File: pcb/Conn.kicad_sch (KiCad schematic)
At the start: 5 parts

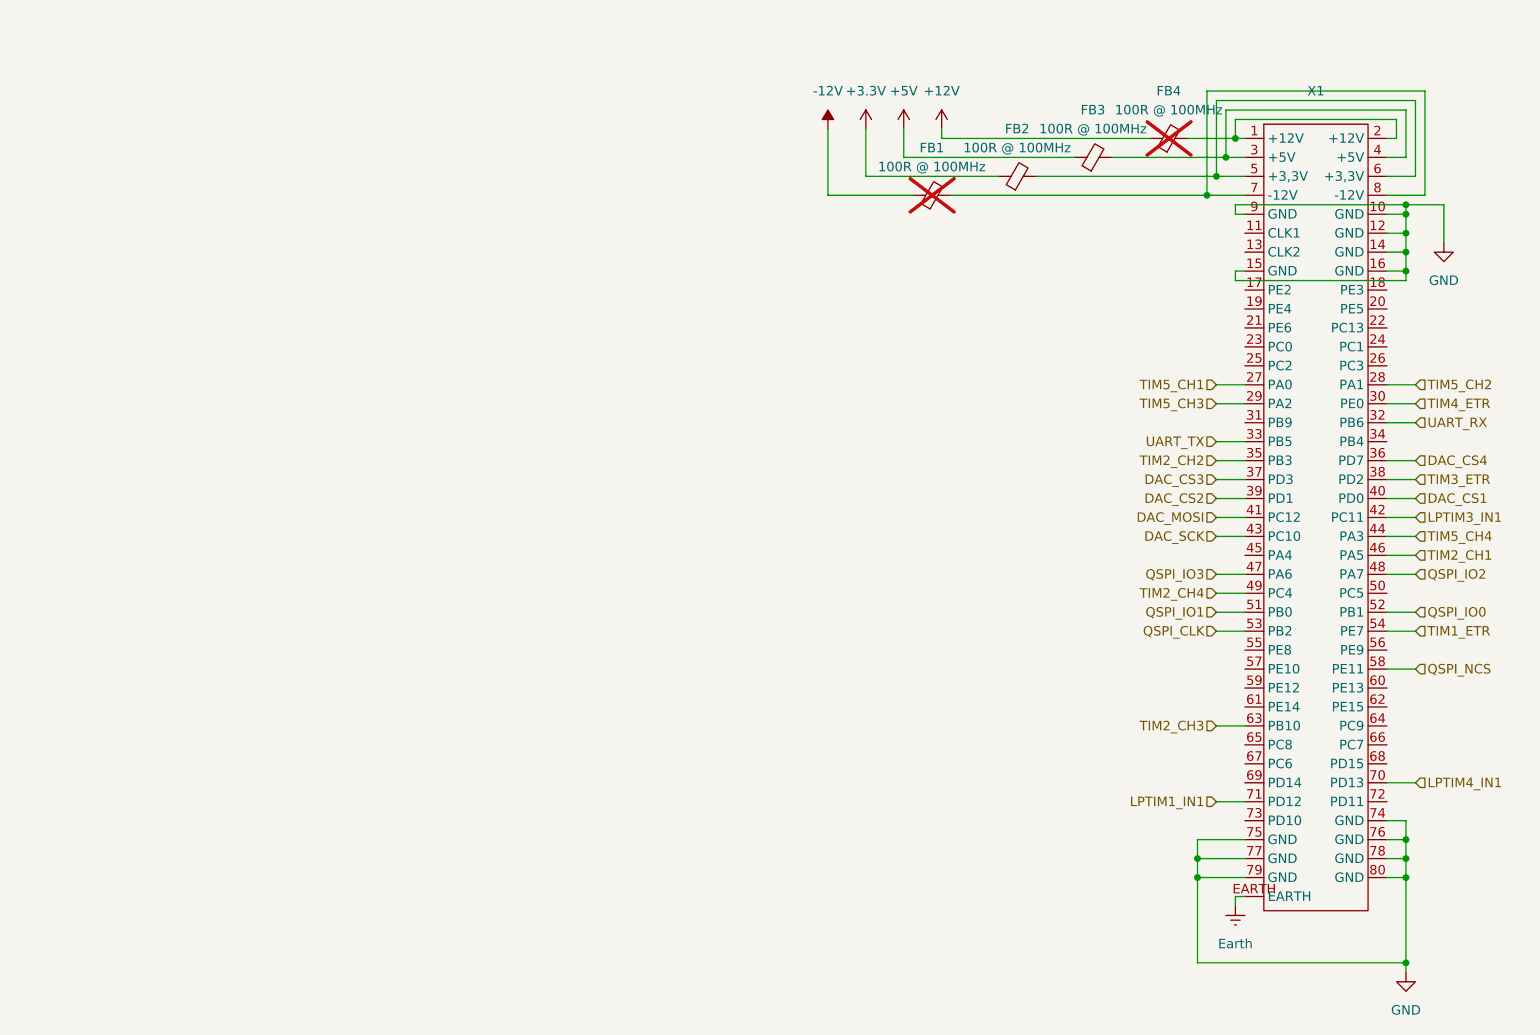
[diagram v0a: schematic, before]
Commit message: Cleaning
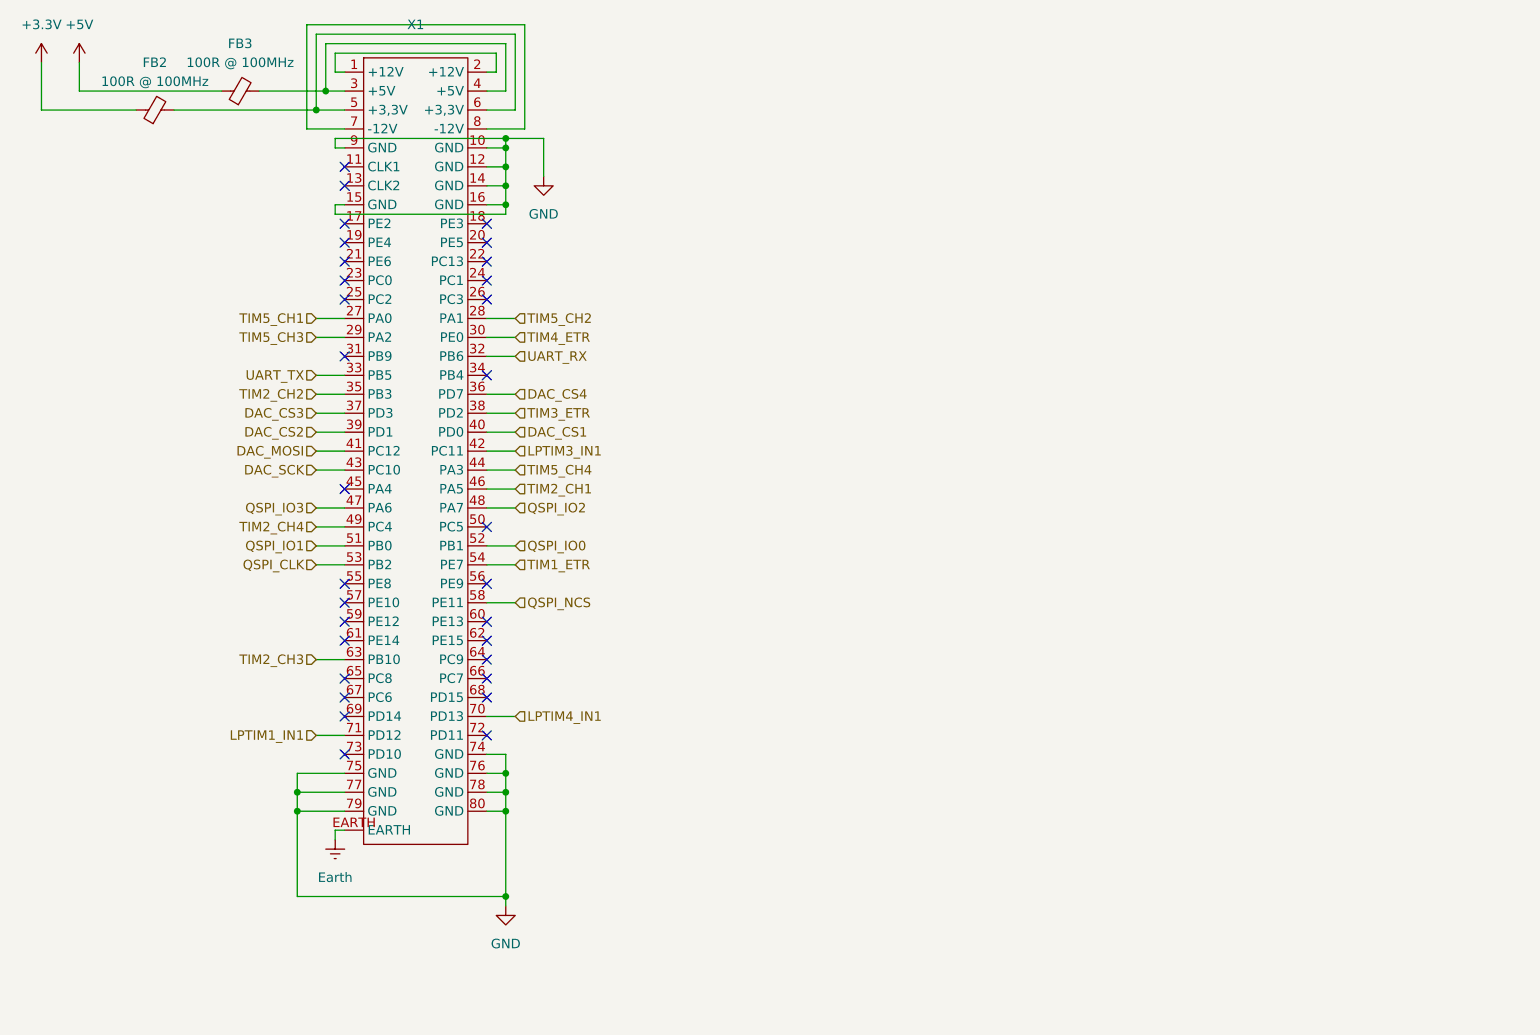
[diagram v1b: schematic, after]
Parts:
- removed FB1, FB4: 100R @ 100MHz, Inductor_SMD:L_0603_1608Metric, symbol Device:FerriteBead_Small
- FB2, FB3: Manufacturer_Part_Number (none) -> WLBD1608HCU101TL
- X1: value ~ -> (none); now left out of the parts list
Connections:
- no-connect marks 0 -> 31
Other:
- moved on the sheet: FB2, FB3, X1
